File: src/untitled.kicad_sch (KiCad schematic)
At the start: 47 parts, among them J5 USB_C_Receptacle_USB2.0_14P, J6 Conn_02x26_Odd_Even, J7 SM03B-SRSS-TB, J8 Conn_02x26_Odd_Even, U4 W25Q128JVS, U5 NCP1117-1.5_SOT223, Y2 ABM8-272-T3

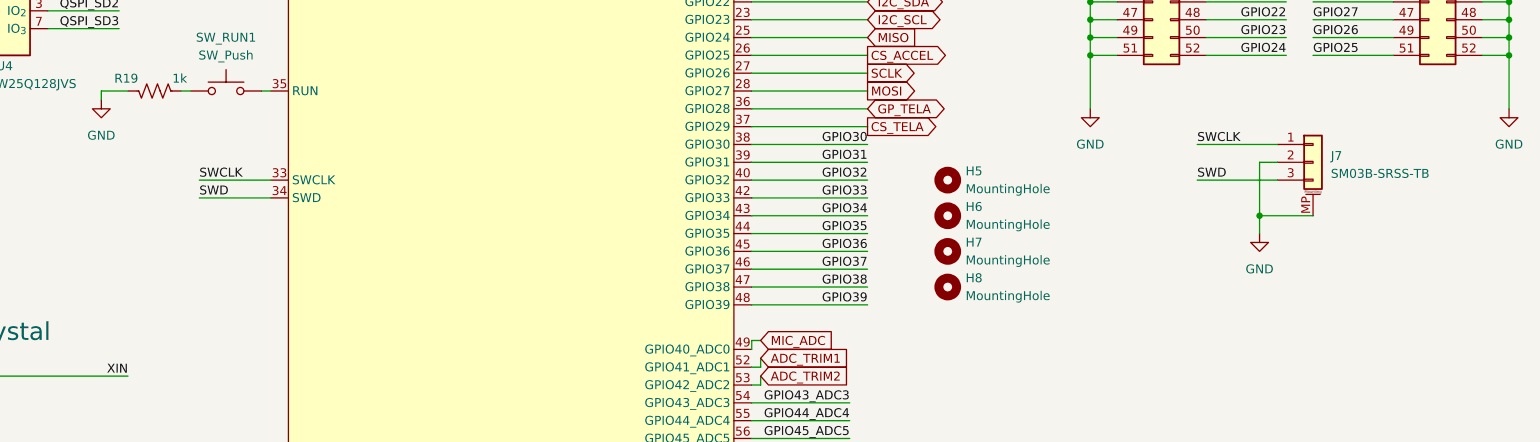
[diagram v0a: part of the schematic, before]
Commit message: revisão da RP2040
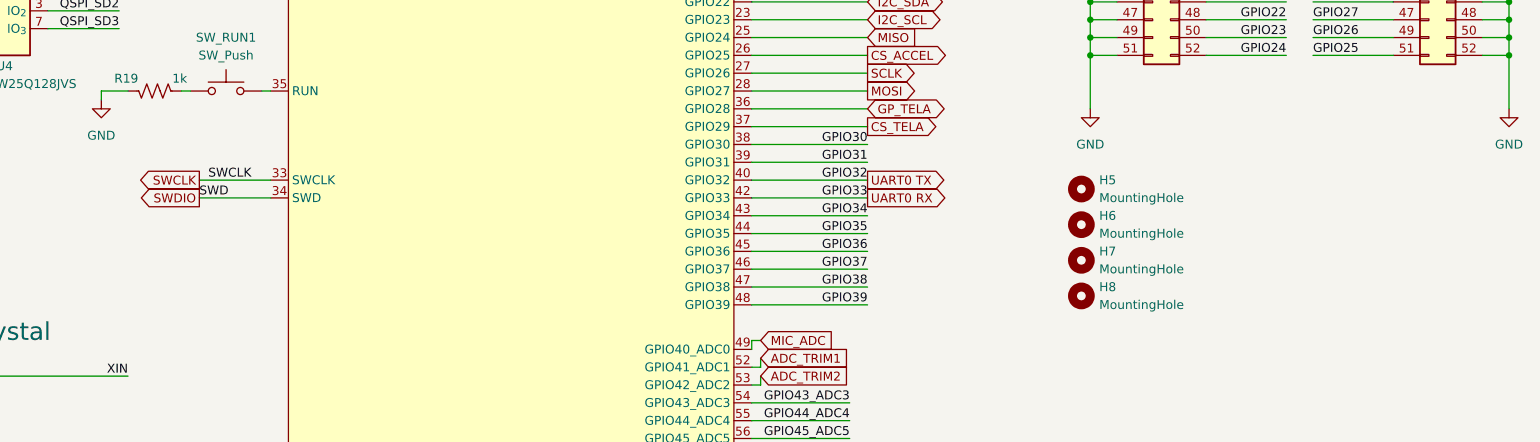
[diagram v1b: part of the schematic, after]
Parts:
- removed J7: SM03B-SRSS-TB, Connector_JST:JST_SH_SM03B-SRSS-TB_1x03-1MP_P1.00mm_Horizontal, symbol Connector_Generic_MountingPin:Conn_01x03_MountingPin
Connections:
- net GPIO32 renamed UART0 TX
- net GPIO33 renamed UART0 RX
- net SWD renamed SWDIO
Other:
- moved on the sheet: H5, H6, H7, H8
